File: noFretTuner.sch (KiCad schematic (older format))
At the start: 4 parts, among them J1 Microphone Connection, J2 DC Supply Connection, J3 Battery Connection, U1 STM32F091RCT6

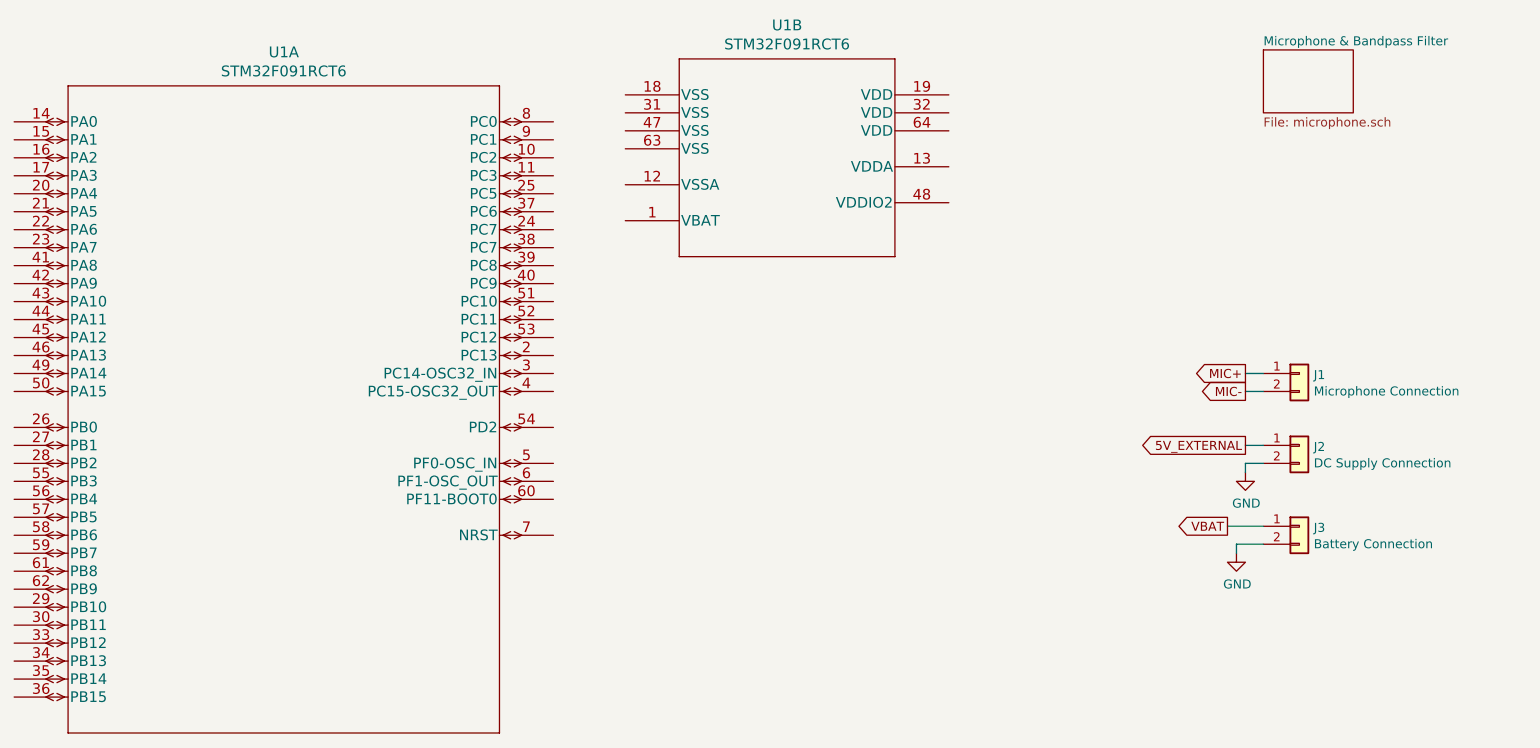
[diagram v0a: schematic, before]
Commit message: Motor Controller Done
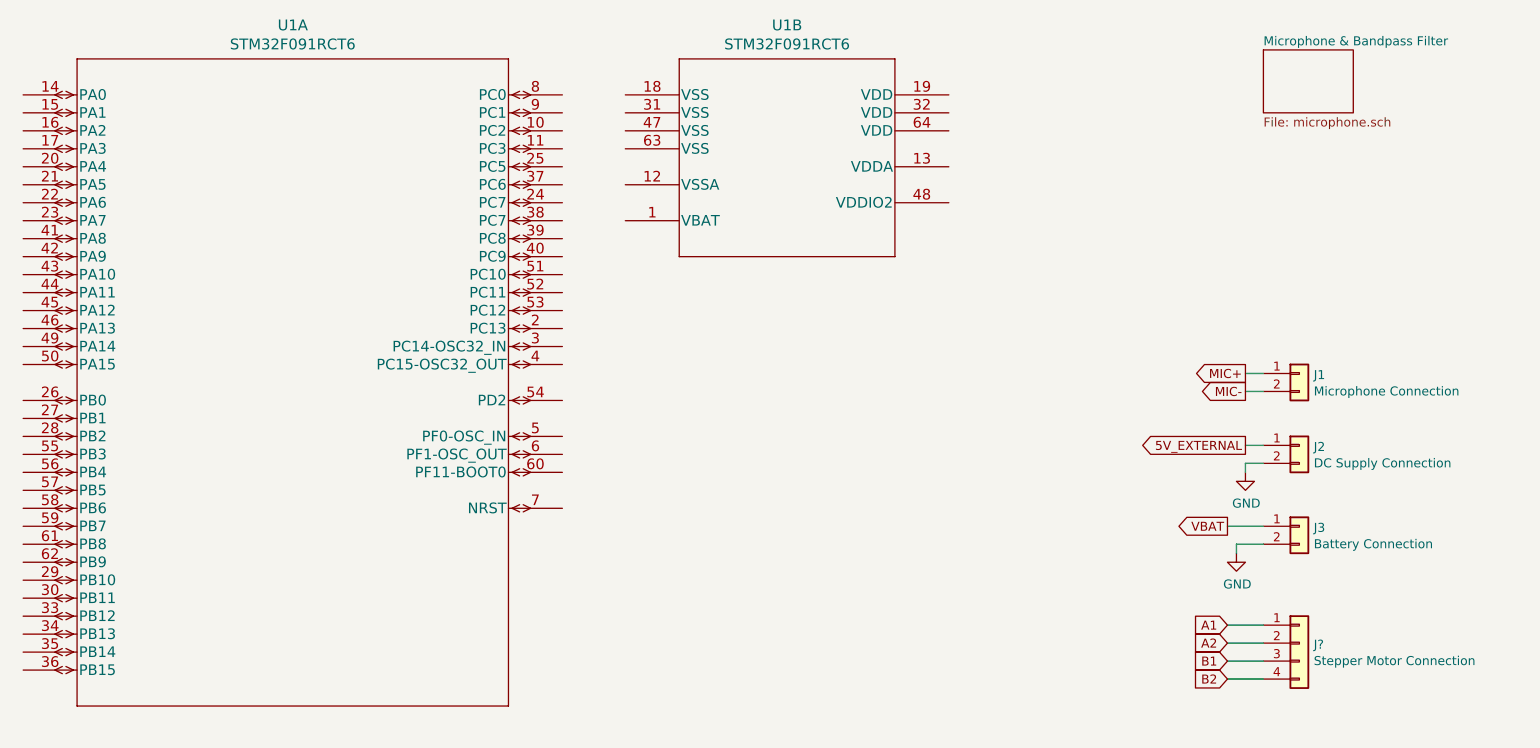
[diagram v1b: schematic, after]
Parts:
- added J?: Stepper Motor Connection, symbol Connector_Generic:Conn_01x04
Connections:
- new net A1: J?.1 (Pin_1)
- new net A2: J?.2 (Pin_2)
- new net B1: J?.3 (Pin_3)
- new net B2: J?.4 (Pin_4)
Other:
- moved on the sheet: U1A
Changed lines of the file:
@@
-$Comp
-L STM32F091RCT6:STM32F091RCT6 U1
-U 1 1 62040D0D
-P 750 1100
-F 0 "U1" H 2250 1487 60  0000 C CNN
-F 1 "STM32F091RCT6" H 2250 1381 60  0000 C CNN
-F 2 "LQFP64-10x10mm" H 1650 1340 60  0001 C CNN
-F 3 "" H 750 1100 60  0000 C CNN
-	1    750  1100
-	1    0    0    -1
-$EndComp
 $Comp
 L STM32F091RCT6:STM32F091RCT6 U1
@@
 F 3 "" H 4150 950 60  0000 C CNN
 	2    4150 950
-	1    0    0    -1
-$EndComp
-$Sheet
-S 7700 700  500  350
-U 6207A6E4
-F0 "Microphone & Bandpass Filter" 50
-F1 "microphone.sch" 50
-$EndSheet
-$Comp
-L Connector_Generic:Conn_01x02 J1
-U 1 1 620A7E14
-P 7900 2500
-F 0 "J1" H 7980 2492 50  0000 L CNN
-F 1 "Microphone Connection" H 7980 2401 50  0000 L CNN
-F 2 "TerminalBlock_TE-Connectivity:TerminalBlock_TE_282834-2_1x02_P2.54mm_Horizontal" H 7900 2500 50  0001 C CNN
-F 3 "~" H 7900 2500 50  0001 C CNN
-	1    7900 2500
 	1    0    0    -1
 $EndComp
@@
 Wire Wire Line
 	7600 3000 7600 3050
+$Comp
+L Connector_Generic:Conn_01x02 J1
+U 1 1 620A7E14
+P 7900 2500
+F 0 "J1" H 7980 2492 50  0000 L CNN
+F 1 "Microphone Connection" H 7980 2401 50  0000 L CNN
+F 2 "TerminalBlock_TE-Connectivity:TerminalBlock_TE_282834-2_1x02_P2.54mm_Horizontal" H 7900 2500 50  0001 C CNN
+F 3 "~" H 7900 2500 50  0001 C CNN
+	1    7900 2500
+	1    0    0    -1
+$EndComp
+$Sheet
+S 7700 700  500  350
+U 6207A6E4
+F0 "Microphone & Bandpass Filter" 50
+F1 "microphone.sch" 50
+$EndSheet
+$Comp
+L STM32F091RCT6:STM32F091RCT6 U1
+U 1 1 62040D0D
+P 800 950
+F 0 "U1" H 2300 1337 60  0000 C CNN
+F 1 "STM32F091RCT6" H 2300 1231 60  0000 C CNN
+F 2 "LQFP64-10x10mm" H 1700 1190 60  0001 C CNN
+F 3 "" H 800 950 60  0000 C CNN
+	1    800  950
+	1    0    0    -1
+$EndComp
+$Comp
+L Connector_Generic:Conn_01x04 J?
+U 1 1 623ABF0F
+P 7900 4000
+F 0 "J?" H 7980 3992 50  0000 L CNN
+F 1 "Stepper Motor Connection" H 7980 3901 50  0000 L CNN
+F 2 "" H 7900 4000 50  0001 C CNN
+F 3 "~" H 7900 4000 50  0001 C CNN
+	1    7900 4000
+	1    0    0    -1
+$EndComp
+Text GLabel 7500 3900 0    50   Input ~ 0
+A1
+Text GLabel 7500 4000 0    50   Input ~ 0
+A2
+Text GLabel 7500 4100 0    50   Input ~ 0
+B1
+Text GLabel 7500 4200 0    50   Input ~ 0
+B2
+Wire Wire Line
+	7500 3900 7700 3900
+Wire Wire Line
+	7500 4000 7700 4000
+Wire Wire Line
+	7500 4100 7700 4100
+Wire Wire Line
+	7500 4200 7700 4200
 $EndSCHEMATC

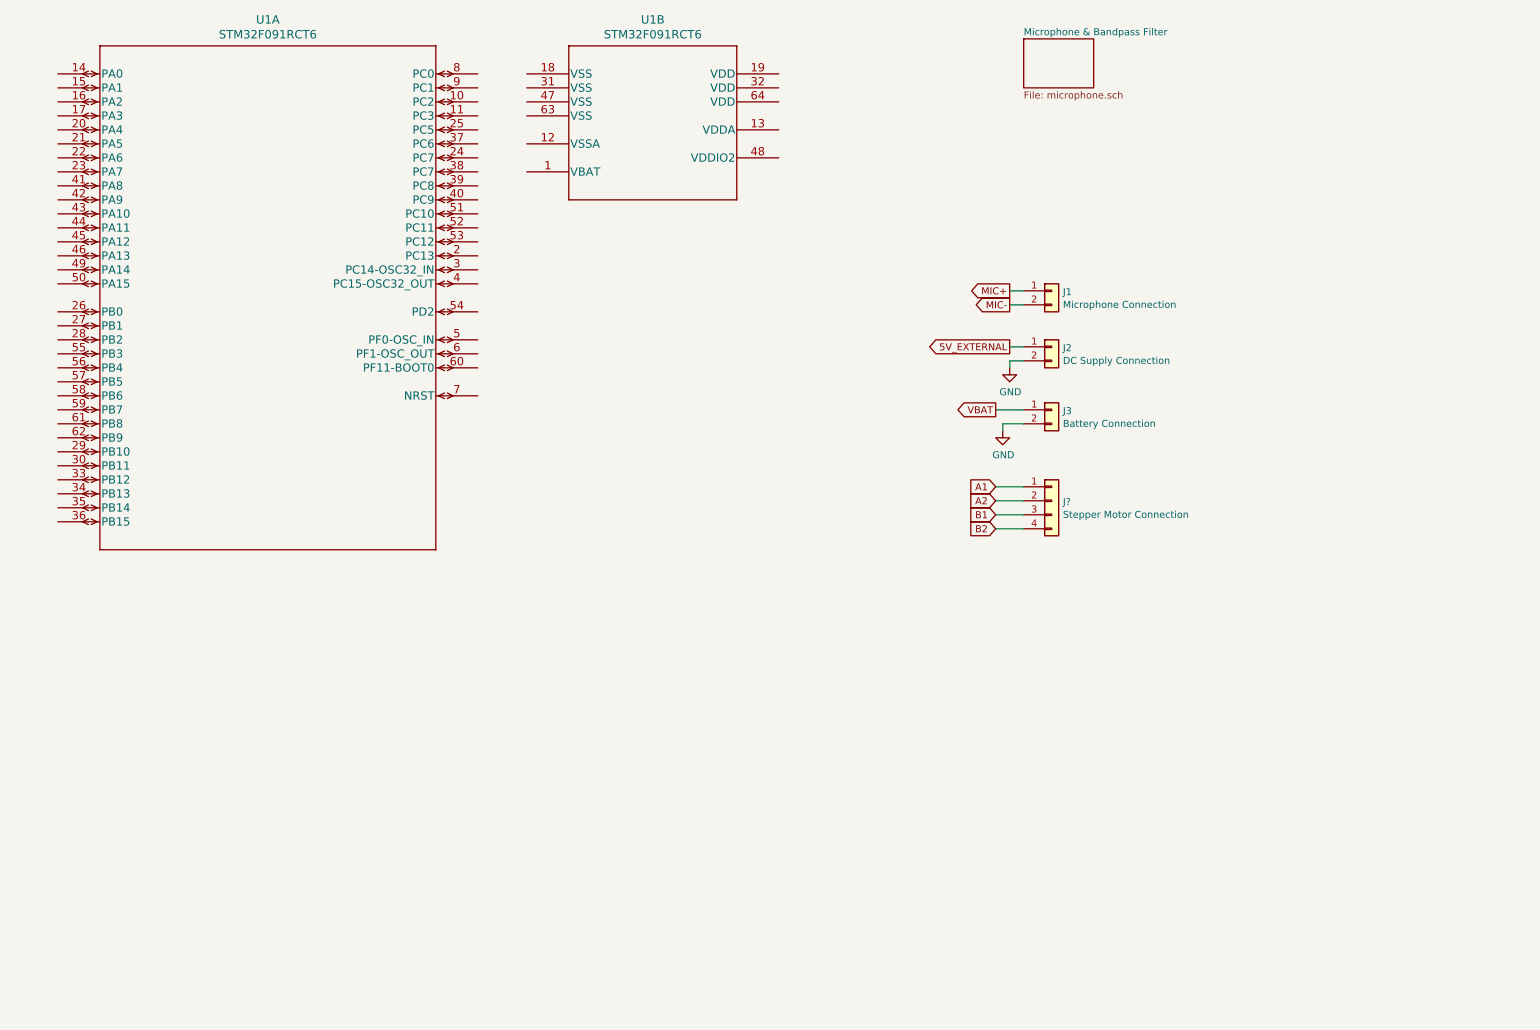
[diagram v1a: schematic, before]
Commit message: First Draft Complete
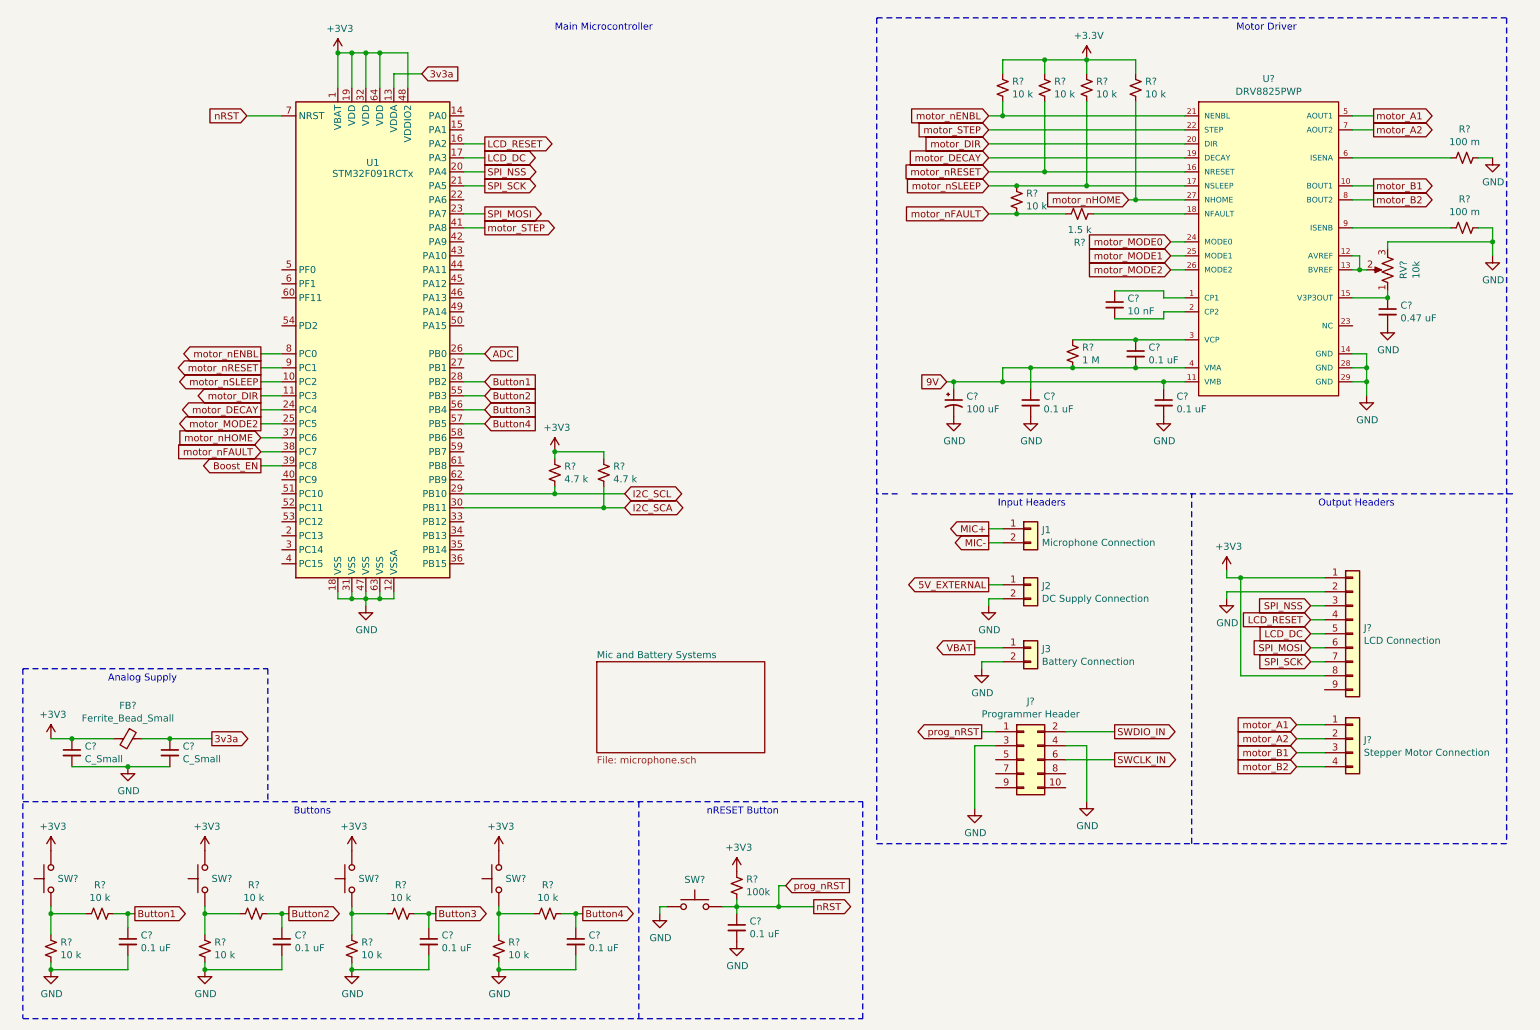
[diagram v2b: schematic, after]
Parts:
- removed U1: STM32F091RCT6, LQFP64-10x10mm, symbol STM32F091RCT6:STM32F091RCT6
- added C? (x2): C_Small, symbol Device:C_Small
- added C? (x8): 0.1 uF, symbol Device:C_Small
- added C?: 100 uF, symbol Device:CP1_Small
- added C?: 10 nF, symbol Device:C_Small
- added C?: 0.47 uF, symbol Device:C_Small
- added FB?: Ferrite_Bead_Small, symbol Device:Ferrite_Bead_Small
- added J?: Programmer Header, symbol Connector_Generic:Conn_02x05_Odd_Even
- added J?: LCD Connection, symbol Connector_Generic:Conn_01x09
- added R? (x8): 10 k, symbol Device:R_Small_US
- added R? (x2): 4.7 k, symbol Device:R_Small_US
- added R?: 100k, symbol Device:R_Small_US
- added R?: 1 M, Resistor_SMD:R_0805_2012Metric_Pad1.15x1.40mm_HandSolder, symbol Device:R_Small_US
- added R? (x2): 100 m, Resistor_SMD:R_0805_2012Metric_Pad1.15x1.40mm_HandSolder, symbol Device:R_Small_US
- added R? (x5): 10 k, Resistor_SMD:R_0805_2012Metric_Pad1.15x1.40mm_HandSolder, symbol Device:R_Small_US
- added R?: 1.5 k, Resistor_SMD:R_0805_2012Metric_Pad1.15x1.40mm_HandSolder, symbol Device:R_Small_US
- added RV?: 10k, symbol Device:R_POT_US
- added SW? (x5): Switch_SW_Push, symbol STM32F091RCTx:Switch_SW_Push
- added U1: STM32F091RCTx, Package_QFP:LQFP-64_10x10mm_P0.5mm, symbol STM32F091RCTx:STM32F091RCTx
- added U?: DRV8825PWP, Texas_Instruments-DRV8825PWP-*, symbol DRV8825PWP:DRV8825PWP
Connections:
- net GND: now also C?.2, C?.2, C?.2, C?.2, C?.2, C?.2, C?.2, C?.2, C?.2, C?.2, C?.2, J?.2 (Pin_2), J?.3 (Pin_3), J?.4 (Pin_4), R?.1, R?.1, R?.2, R?.2, R?.2, R?.2, RV?.3, SW?.1, U1.12 (VSSA), U1.18 (VSS), U1.31 (VSS), U1.47 (VSS), U1.63 (VSS), U?.14 (GND), U?.28 (GND), U?.29 (GND)
- net A1 renamed motor_A1
- net motor_A1: now also U?.5 (AOUT1)
- net A2 renamed motor_A2
- net motor_A2: now also U?.7 (AOUT2)
- net B1 renamed motor_B1
- net motor_B1: now also U?.10 (BOUT1)
- net B2 renamed motor_B2
- net motor_B2: now also U?.8 (BOUT2)
- new net: R?.1, R?.2, SW?.1 (x4)
- new net: C?.1, R?.1, U?.3 (VCP)
- new net: C?.1, U?.1 (CP1)
- new net: C?.2, U?.2 (CP2)
- new net: R?.2, U?.6 (ISENA)
- new net: C?.1, RV?.1, U?.15 (V3P3OUT)
- new net: RV?.2, U?.12 (AVREF), U?.13 (BVREF)
- new net: R?.2, U?.18 (NFAULT)
- new net: R?.2, U?.9 (ISENB)
- new net +3V3: C?.1, FB?.2, J?.1 (Pin_1), J?.8 (Pin_8), R?.1, R?.1, R?.1, R?.1, R?.1, R?.1, R?.1, SW?.2, SW?.2, SW?.2, SW?.2, U1.1 (VBAT), U1.19 (VDD), U1.32 (VDD), U1.48 (VDDIO2), U1.64 (VDD)
- new net 3v3a: C?.1, FB?.1, U1.13 (VDDA)
- new net 9V: C?.1, C?.1, C?.1, C?.2, R?.2, U?.11 (VMB), U?.4 (VMA)
- new net ADC: U1.26 (PB0)
- new net Boost_EN: U1.39 (PC8)
- new net Button1: C?.1, R?.1, U1.28 (PB2)
- new net Button2: C?.1, R?.1, U1.55 (PB3)
- new net Button3: C?.1, R?.1, U1.56 (PB4)
- new net Button4: C?.1, R?.1, U1.57 (PB5)
- new net I2C_SCA: R?.2, U1.30 (PB11)
- new net I2C_SCL: R?.2, U1.29 (PB10)
- new net LCD_DC: J?.5 (Pin_5), U1.17 (PA3)
- new net LCD_RESET: J?.4 (Pin_4), U1.16 (PA2)
- new net SPI_MOSI: J?.6 (Pin_6), U1.23 (PA7)
- new net SPI_NSS: J?.3 (Pin_3), U1.20 (PA4)
- new net SPI_SCK: J?.7 (Pin_7), U1.21 (PA5)
- new net SWCLK_IN: J?.6 (Pin_6)
- new net SWDIO_IN: J?.2 (Pin_2)
- new net motor_DECAY: U1.24 (PC4), U?.19 (DECAY)
- new net motor_DIR: U1.11 (PC3), U?.20 (DIR)
- new net motor_MODE0: U?.24 (MODE0)
- new net motor_MODE1: U?.25 (MODE1)
- new net motor_MODE2: U1.25 (PC5), U?.26 (MODE2)
- new net motor_STEP: U1.41 (PA8), U?.22 (STEP)
- new net motor_nENBL: R?.2, U1.8 (PC0), U?.21 (NENBL)
- new net motor_nFAULT: R?.1, R?.2, U1.38 (PC7)
- new net motor_nHOME: R?.2, U1.37 (PC6), U?.27 (NHOME)
- new net motor_nRESET: R?.2, U1.9 (PC1), U?.16 (NRESET)
- new net motor_nSLEEP: R?.1, R?.2, U1.10 (PC2), U?.17 (NSLEEP)
- new net nRST: C?.1, J?.1 (Pin_1), R?.2, SW?.2, U1.7 (NRST)
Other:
- note added: "Analog Supply"
- note added: "Buttons"
- note added: "Input Headers"
- note added: "Main Microcontroller"
- note added: "Motor Driver"
- note added: "Output Headers"
- note added: "nRESET Button"
- moved on the sheet: J1, J2, J3, J?

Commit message: Oscillator and Decouple Caps
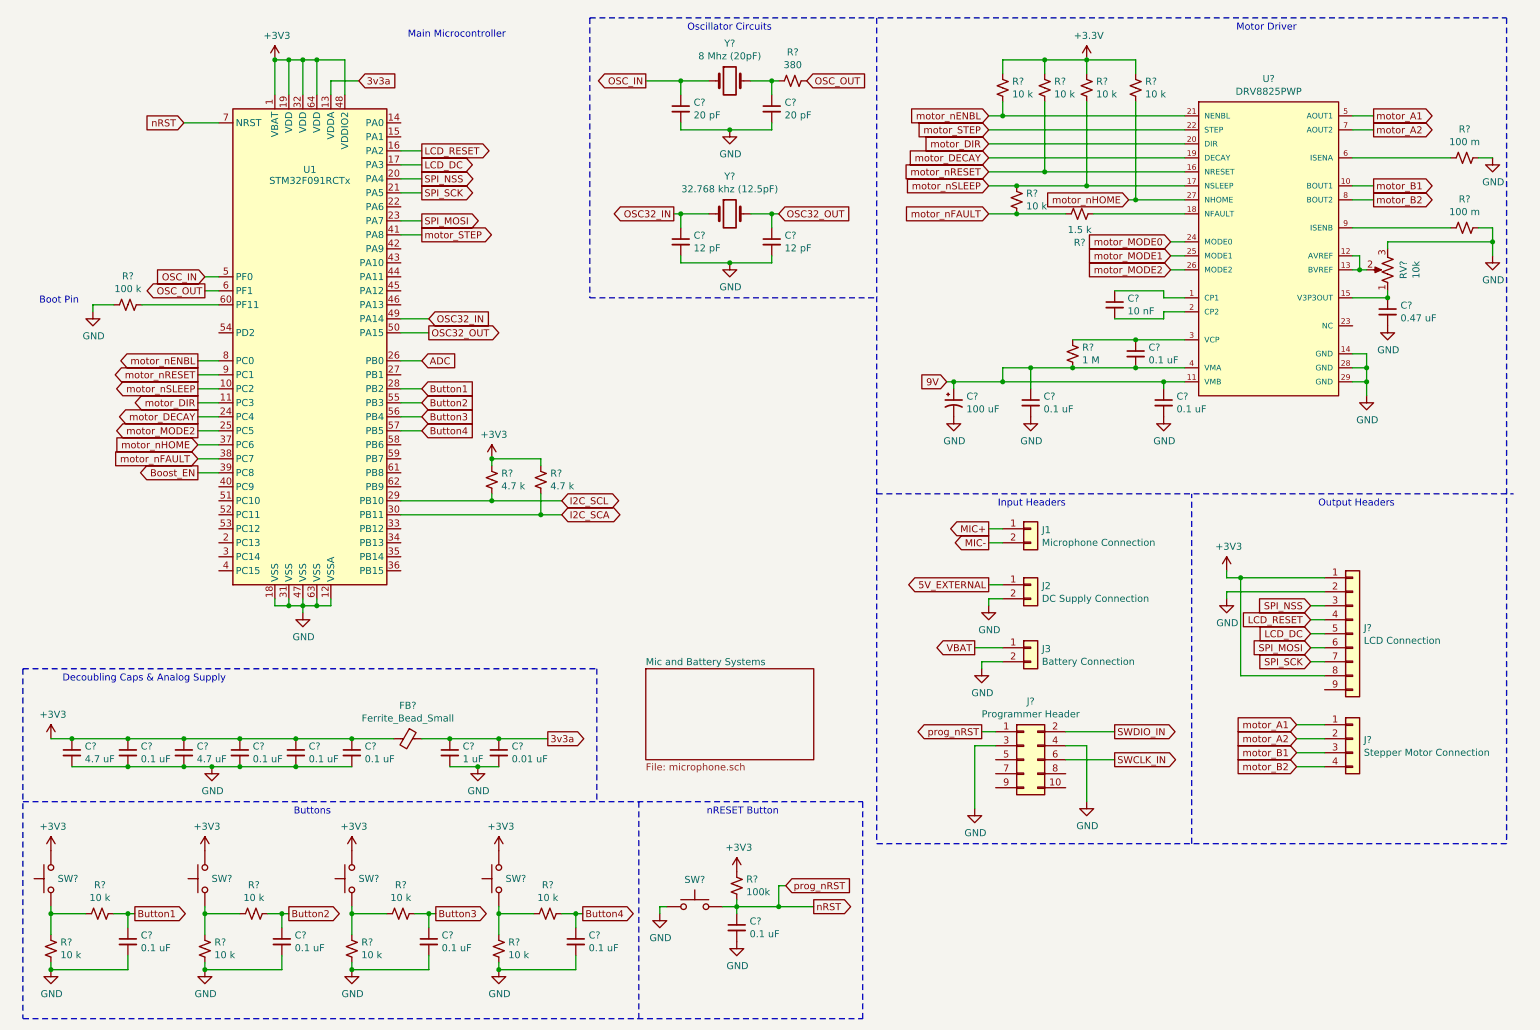
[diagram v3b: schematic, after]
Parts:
- added C? (x4): 0.1 uF, symbol Device:C_Small
- added C?: 4.7 uF, symbol Device:C_Small
- added C?: 0.01 uF, symbol Device:C_Small
- added C? (x2): 12 pF, symbol Device:C_Small
- added C? (x2): 20 pF, symbol Device:C_Small
- added R?: 100 k, symbol Device:R_Small_US
- added R?: 380, symbol Device:R_Small_US
- added Y?: 32.768 khz (12.5pF), symbol Device:Crystal
- added Y?: 8 Mhz (20pF), symbol Device:Crystal
- C?: value C_Small -> 1 uF
- C?: value C_Small -> 4.7 uF
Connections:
- net +3V3: now also C?.1, C?.1, C?.1, C?.1, C?.1
- net 3v3a: now also C?.1
- net GND: now also C?.2, C?.2, C?.2, C?.2, C?.2, C?.2, C?.2, C?.2, C?.2, C?.2, R?.2
- net OSC32_IN: now reaches U1.49 (PA14)
- net OSC32_IN: now also C?.1, Y?.1
- net OSC_IN: now reaches U1.5 (PF0)
- net OSC_IN: now also C?.1, Y?.1
- net OSC32_OUT: now reaches U1.50 (PA15)
- net OSC32_OUT: now also C?.1, Y?.2
- net OSC_OUT: now reaches U1.6 (PF1)
- net OSC_OUT: now also R?.1
- net at U1.60 (PF11): now also R?.1
- new net: C?.1, R?.2, Y?.2
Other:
- note added: "Boot Pin"
- note added: "Decoubling Caps & Analog Supply"
- note added: "Oscillator Circuits"
- note removed: "Analog Supply"
- moved on the sheet: C?, FB?, R?, U1
